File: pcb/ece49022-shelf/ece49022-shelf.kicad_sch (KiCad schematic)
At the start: 0 parts

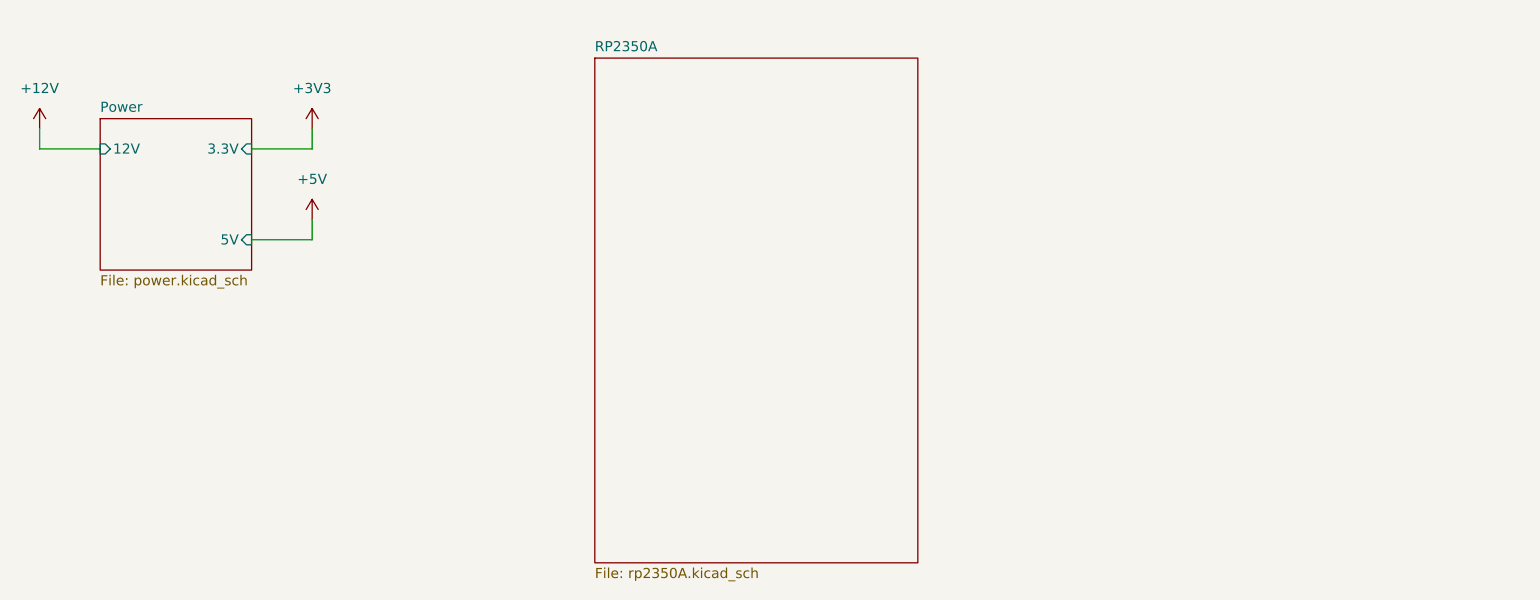
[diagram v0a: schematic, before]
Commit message: updated schematic
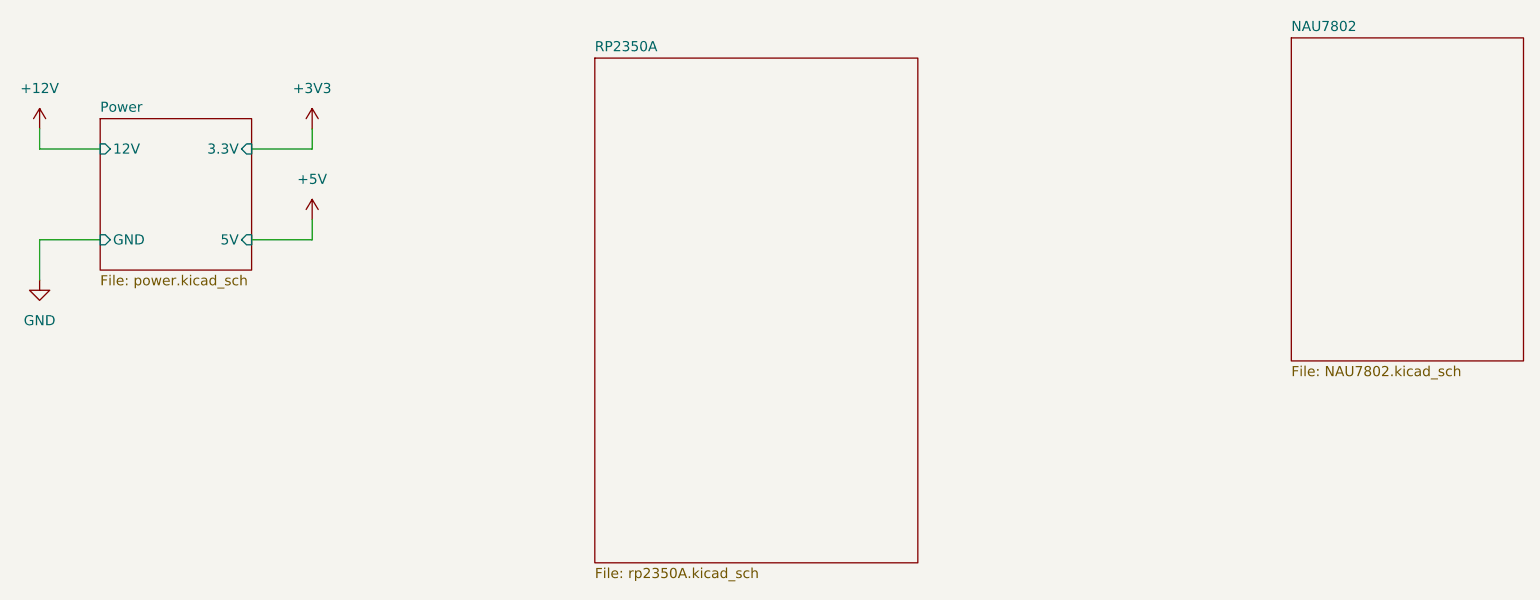
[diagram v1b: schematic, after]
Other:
- added sheet NAU7802 (NAU7802.kicad_sch)
- sheet Power ports: added GND; removed none
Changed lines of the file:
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@@
+	(wire
+		(pts
+			(xy 25.4 97.79) (xy 25.4 102.87)
+		)
+		(stroke
+			(width 0)
+			(type default)
+		)
+	)
 	(wire
 		(pts
@@
 		(pts
 			(xy 25.4 83.82) (xy 25.4 86.36)
+		)
+		(stroke
+			(width 0)
+			(type default)
+		)
+	)
+	(wire
+		(pts
+			(xy 33.02 97.79) (xy 25.4 97.79)
 		)
 		(stroke
@@
 	)
 	(symbol
+		(lib_id "power:GND")
+		(at 25.4 102.87 0)
+		(unit 1)
+		(exclude_from_sim no)
+		(in_bom yes)
+		(on_board yes)
+		(dnp no)
+		(fields_autoplaced yes)
+		(property "Reference" "#PWR015"
+			(at 25.4 109.22 0)
+			(effects
+				(font
+					(size 1.27 1.27)
+				)
+				(hide yes)
+			)
+		)
+		(property "Value" "GND"
+			(at 25.4 107.95 0)
+			(effects
+				(font
+					(size 1.27 1.27)
+				)
+			)
+		)
+		(property "Footprint" ""
+			(at 25.4 102.87 0)
+			(effects
+				(font
+					(size 1.27 1.27)
+				)
+				(hide yes)
+			)
+		)
+		(property "Datasheet" ""
+			(at 25.4 102.87 0)
+			(effects
+				(font
+					(size 1.27 1.27)
+				)
+				(hide yes)
+			)
+		)
+		(property "Description" "Power symbol creates a global label with name \"GND\" , ground"
+			(at 25.4 102.87 0)
+			(effects
+				(font
+					(size 1.27 1.27)
+				)
+				(hide yes)
+			)
+		)
+		(pin "1"
+		)
+		(instances
+			(project ""
+				(path "/cb6cb1b4-c151-4aa2-8cd7-5430288cfa02"
+					(reference "#PWR015")
+					(unit 1)
+				)
+			)
+		)
+	)
+	(symbol
 		(lib_id "power:+5V")
 		(at 59.69 95.25 0)
@@
 			)
 		)
+		(pin "GND" input
+			(at 33.02 97.79 180)
+			(effects
+				(font
+					(size 1.27 1.27)
+				)
+				(justify left)
+			)
+		)
 		(instances
 			(project "ece49022-shelf"
@@
 				)
 			)
+		)
+	)
+	(sheet
+		(at 182.88 72.39)
+		(size 29.21 40.64)
+		(exclude_from_sim no)
+		(in_bom yes)
+		(on_board yes)
+		(dnp no)
+		(fields_autoplaced yes)
+		(stroke
+			(width 0.1524)
+			(type solid)
+		)
+		(fill
+			(color 0 0 0 0.0000)
+		)
+		(property "Sheetname" "NAU7802"
+			(at 182.88 71.6784 0)
+			(effects
+				(font
+					(size 1.27 1.27)
+				)
+				(justify left bottom)
+			)
+		)
+		(property "Sheetfile" "NAU7802.kicad_sch"
+			(at 182.88 113.6146 0)
+			(effects
+				(font
+					(size 1.27 1.27)
+				)
+				(justify left top)
+			)
+		)
+		(instances
+			(project "ece49022-shelf"
+				(path "/cb6cb1b4-c151-4aa2-8cd7-5430288cfa02"
+					(page "4")
+				)
+			)
